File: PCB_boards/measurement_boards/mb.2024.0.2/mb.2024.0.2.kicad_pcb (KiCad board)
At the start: 2 copper layers, 247.8 x 124.2 mm, 121 parts, among them J1 DSP_out_12v_GND, J10 DSP+, J11 Screw_Terminal_VMN, J12 Conn_01x08_Female, J13 Connector_I2C_for_mux, J14 Conn_01x02_Female, J15 Conn_01x08_Female, J16 RX_bat, J17 DSP GND, J18 ELEC_M, J19 ELEC_N, J2 DPS5005_input_0_to_50V, J20 shunt +, J21 shunt -, J22 Conn_01x04_Female, J23 Conn_01x05_Female, J24 Connector_I2C_for_MC, J25 Conn_01x04_Female, J26 Conn_01x05_Female, J3 Screw_Terminal_AB, J4 Conn_01x08_Female, J5 Conn_01x04_Female, J6 Conn_01x08_Female, J7 Raspberry_Pi_2_3, J8 Connector_I2C_for_MCP23008, J9 TX_bat, K1 G5LE-1, K2 G5LE-1, K3 G5LE-1, K4 G5LE-1, K5 G5LE-1, K6 G5LE-1, Q1 ZVN4206ASTZ, Q2 ZVN4206ASTZ, Q3 ZVN4206ASTZ, Q4 ZVN4206ASTZ, Q5 ZVN4206ASTZ, Q6 ZVN4206ASTZ, U1 MCP23008-xP, U10 DG411xJ, U2 OP07, U3 24LC02, U4 1085, U5 1085, U6 OP07, U7 REF03GP, U8 MCP23008-xP, U9 OP07

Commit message: correction DPS, add dischage resistor, remove 63 warning on the schemtic, remove 7 errors in schematics change resistor designation, update pcb
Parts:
- removed C9: 10uF, Capacitor_THT:CP_Radial_D6.3mm_P2.50mm
- removed LED10-OHMPI-MEASURE: LED, LED_THT:LED_D4.0mm
- removed R11: 330 ohms, Resistor_THT:R_Axial_DIN0207_L6.3mm_D2.5mm_P7.62mm_Horizontal
- removed R21, R22: 4.7K, Resistor_THT:R_Axial_DIN0207_L6.3mm_D2.5mm_P7.62mm_Horizontal
- added C5: 10uF, Capacitor_THT:CP_Radial_D6.3mm_P2.50mm, F.Cu at (109.3, 81.5)
- added D9: 1N4001, Diode_THT:D_DO-41_SOD81_P10.16mm_Horizontal, F.Cu at (153.4, 127.3)
- added J27: Screw_Terminal_01x03, TerminalBlock:TerminalBlock_bornier-3_P5.08mm, F.Cu at (105.2, 51.1)
- added K7: G5LE-1, Relay_THT:Relay_SPDT_Omron-G5LE-1, F.Cu at (168.6, 132.1)
- added Q7: ZVN4206ASTZ, Package_TO_SOT_THT:TO-92L_Wide, F.Cu at (188.5, 135.9)
- added R8: 1k, Resistor_THT:R_Axial_DIN0207_L6.3mm_D2.5mm_P7.62mm_Horizontal, F.Cu at (156.7, 131.6)
- added R9: 100k, Resistor_THT:R_Axial_DIN0207_L6.3mm_D2.5mm_P7.62mm_Horizontal, F.Cu at (195.3, 142.5)
- J1: value DSP_out_12v_GND -> DPS_out_12v_GND
- J10: value DSP+ -> DPS+
- J12, J15, J4, J6: value Conn_01x08_Female -> Conn_01x08_Socket
- J14: value Conn_01x02_Female -> Conn_01x02_Socket
- J17: value DSP GND -> DPS GND
- J22: renamed from J5; value Conn_01x04_Female -> Conn_01x04_Socket
- J23: renamed from J26; value Conn_01x05_Female -> Conn_01x05_Socket
- J25: renamed from J22; value Conn_01x04_Female -> Conn_01x04_Socket
- J26: renamed from J23; value Conn_01x05_Female -> Conn_01x05_Socket
- J5: renamed from J25; value Conn_01x04_Female -> Conn_01x04_Socket
- moved J21 9.45 mm to (160.8, 141.0)
- renumbered D9 to D3, D10 to D4, D11 to D7, D12 to D8, LED11-OHMPI-STACK to LED11-OHMPI-STACK1, LED12-LOW-TX-BATTERY to LED12-LOW-TX-BATTERY1, LED9-OHMPI-RUN to LED9-OHMPI-RUN-1
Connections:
- net /Current_injection_and_measurement/Input_DSP_+_alim renamed /Current_injection_and_measurement/Input_DPS_+_alim
- net /Current_injection_and_measurement/Input_DSP_GND_alim renamed /Current_injection_and_measurement/Input_DPS_GND_alim
- net /Relay_switch_dsp/out_12v_DSP renamed /Relay_switch_DPS/out_12v_DPS
- net /Relay_switch_dsp/out_GND_DSP renamed /Relay_switch_DPS/out_GND_DPS
- U4 pad 1: unconnected-(U4-A3-Pad1) -> Net-(J27-Pin_1)
- U4 pad 2: unconnected-(U4-A2-Pad2) -> Net-(J27-Pin_2)
- U4 pad 3: unconnected-(U4-A1-Pad3) -> Net-(J27-Pin_3)
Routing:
- net Net-(J27-Pin_1): track 0.00 -> 43.5 mm
- net Net-(J27-Pin_2): track 0.00 -> 38.9 mm
- net Net-(D9-A): track 0.00 -> 35.8 mm
- net Net-(J27-Pin_3): track 0.00 -> 34.4 mm
- net /Current_injection_and_measurement/Input_DPS_+_alim: track 172.6 -> 199.9 mm
- net 5VD: track 554.0 -> 579.1 mm
- net GP5: track 62.8 -> 84.6 mm
- net Net-(K7-Pad1): track 0.00 -> 12.7 mm
- net GNDD: track 0.00 -> 9.59 mm
- net GP0: track 233.5 -> 225.8 mm
- net AN: track 51.9 -> 59.4 mm
- net GP1: track 282.5 -> 277.0 mm
- net Net-(LED10-OHMPI-MEASURE1-A): track 3.65 -> 0.00 mm
- net /Current_injection_and_measurement/Input_DPS_GND_alim: track 97.0 -> 99.9 mm
- net SDA2: vias 1 -> 2
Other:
- outline, holes or cut-outs redrawn
- board text added: "DPS Input"
- board text added: "DPS out +"
- board text added: "DPS out GND"
- board text removed: "DSP Input"
- board text removed: "Dps out +"
- board text removed: "Dps out GND"

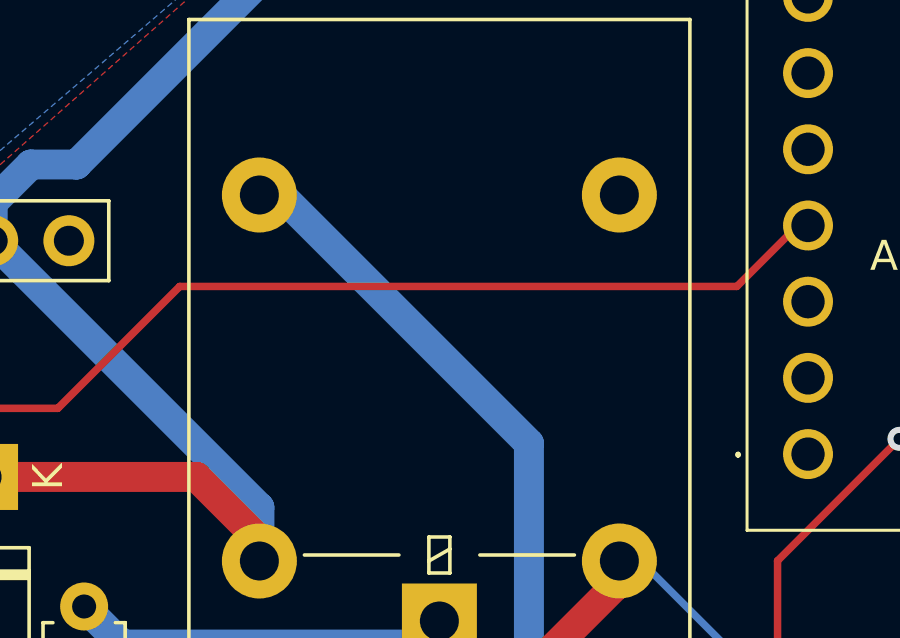
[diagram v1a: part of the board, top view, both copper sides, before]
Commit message: update measurement board
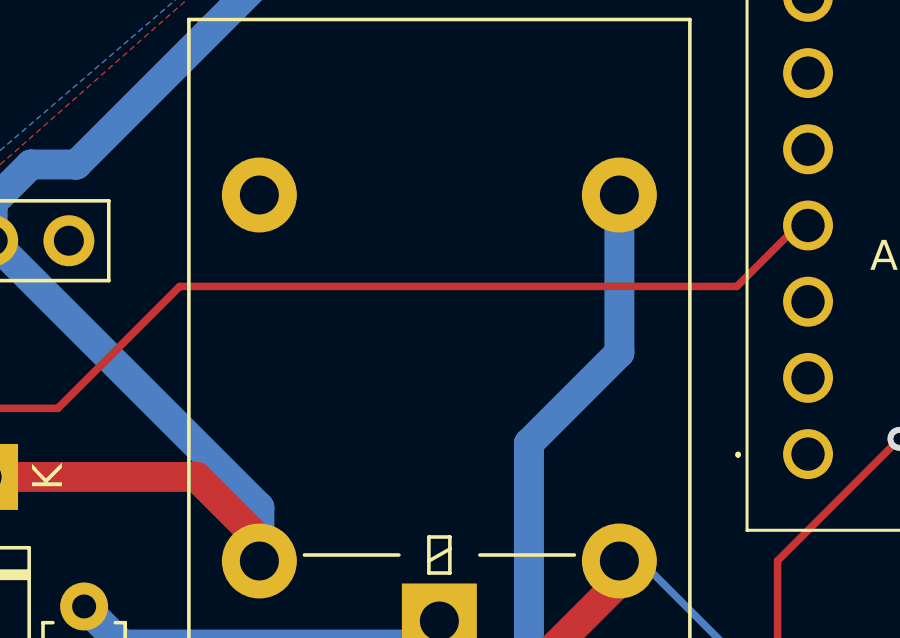
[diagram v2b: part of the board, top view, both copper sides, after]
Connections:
- K7 pad 3: unconnected-(K7-Pad3) -> /Current_injection_and_measurement/Input_DPS_+_alim
- K7 pad 4: /Current_injection_and_measurement/Input_DPS_+_alim -> unconnected-(K7-Pad4)
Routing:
- net /Current_injection_and_measurement/Input_DPS_+_alim: track 199.9 -> 197.0 mm
- net unconnected-(K7-Pad4): track 0.00 -> 0.71 mm
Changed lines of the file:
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@@
   (net 162 "/Current_injection_and_measurement/Input_DPS_GND_alim")
   (net 163 "Net-(K7-Pad1)")
-  (net 164 "unconnected-(K7-Pad3)")
-  (net 165 "Net-(J27-Pin_1)")
-  (net 166 "Net-(J27-Pin_2)")
-  (net 167 "Net-(J27-Pin_3)")
+  (net 164 "Net-(J27-Pin_1)")
+  (net 165 "Net-(J27-Pin_2)")
+  (net 166 "Net-(J27-Pin_3)")
+  (net 167 "unconnected-(K7-Pad4)")
   (footprint "Connector_PinHeader_2.54mm:PinHeader_1x01_P2.54mm_Vertical" (layer "F.Cu")
     (at 26.162 77.978)
@@
       (stroke (width 0.1) (type solid)) (layer "F.Fab"))
     (pad "1" thru_hole rect (at 0 0) (size 3 3) (drill 1.52) (layers "*.Cu" "*.Mask")
-      (net 165 "Net-(J27-Pin_1)") (pinfunction "Pin_1") (pintype "passive"))
+      (net 164 "Net-(J27-Pin_1)") (pinfunction "Pin_1") (pintype "passive"))
     (pad "2" thru_hole circle (at 5.08 0) (size 3 3) (drill 1.52) (layers "*.Cu" "*.Mask")
-      (net 166 "Net-(J27-Pin_2)") (pinfunction "Pin_2") (pintype "passive"))
+      (net 165 "Net-(J27-Pin_2)") (pinfunction "Pin_2") (pintype "passive"))
     (pad "3" thru_hole circle (at 10.16 0) (size 3 3) (drill 1.52) (layers "*.Cu" "*.Mask")
-      (net 167 "Net-(J27-Pin_3)") (pinfunction "Pin_3") (pintype "passive"))
+      (net 166 "Net-(J27-Pin_3)") (pinfunction "Pin_3") (pintype "passive"))
     (model "${KICAD6_3DMODEL_DIR}/TerminalBlock.3dshapes/TerminalBlock_bornier-3_P5.08mm.wrl"
       (offset (xyz 5.079999924 0 0))
@@
     (property "Arrow Part Number" "ZVN4206ASTZ")
     (property "Arrow Price/Stock" "https://www.arrow.com/en/products/zvn4206astz/diodes-incorporated?region=nac")
-    (property "Description" "N-Channel 60 V 600mA (Ta) 700mW (Ta) Through Hole E-Line (TO-92 compatible)")
+    (property "Description" "Transistor JFET - TO shape - relay activation")
     (property "Height" "4.01")
     (property "Manufacturer_Name" "Diodes Incorporated")
@@
       (net 23 "Net-(D9-A)") (pintype "passive"))
     (pad "3" thru_hole oval (at -6 14.2 180) (size 2.5 2.5) (drill 1.3) (layers "*.Cu" "*.Mask")
-      (net 164 "unconnected-(K7-Pad3)") (pintype "passive+no_connect"))
-    (pad "4" thru_hole oval (at 6 14.2 180) (size 2.5 2.5) (drill 1.3) (layers "*.Cu" "*.Mask")
       (net 161 "/Current_injection_and_measurement/Input_DPS_+_alim") (pintype "passive"))
+    (pad "4" thru_hole oval (at 6 14.2 180) (size 2.5 2.5) (drill 1.3) (layers "*.Cu" "*.Mask")
+      (net 167 "unconnected-(K7-Pad4)") (pintype "passive+no_connect"))
     (pad "5" thru_hole oval (at 6 2 180) (size 2.5 2.5) (drill 1.3) (layers "*.Cu" "*.Mask")
       (net 1 "5VD") (pintype "passive"))
@@
       (stroke (width 0.2) (type solid)) (layer "F.Fab"))
     (pad "1" thru_hole circle (at 0 0 270) (size 1.665 1.665) (drill 1.11) (layers "*.Cu" "*.Mask")
-      (net 165 "Net-(J27-Pin_1)") (pinfunction "A3") (pintype "passive"))
+      (net 164 "Net-(J27-Pin_1)") (pinfunction "A3") (pintype "passive"))
     (pad "2" thru_hole circle (at -2.54 0 270) (size 1.665 1.665) (drill 1.11) (layers "*.Cu" "*.Mask")
-      (net 166 "Net-(J27-Pin_2)") (pinfunction "A2") (pintype "passive"))
+      (net 165 "Net-(J27-Pin_2)") (pinfunction "A2") (pintype "passive"))
     (pad "3" thru_hole circle (at -5.08 0 270) (size 1.665 1.665) (drill 1.11) (layers "*.Cu" "*.Mask")
-      (net 167 "Net-(J27-Pin_3)") (pinfunction "A1") (pintype "passive"))
+      (net 166 "Net-(J27-Pin_3)") (pinfunction "A1") (pintype "passive"))
     (pad "4" thru_hole circle (at -7.62 0 270) (size 1.665 1.665) (drill 1.11) (layers "*.Cu" "*.Mask")
       (net 22 "Net-(D5-A)") (pinfunction "A0") (pintype "passive"))
@@
     (property "Arrow Part Number" "ZVN4206ASTZ")
     (property "Arrow Price/Stock" "https://www.arrow.com/en/products/zvn4206astz/diodes-incorporated?region=nac")
-    (property "Description" "N-Channel 60 V 600mA (Ta) 700mW (Ta) Through Hole E-Line (TO-92 compatible)")
+    (property "Description" "Transistor JFET - TO shape - relay activation")
     (property "Height" "4.01")
     (property "Manufacturer_Name" "Diodes Incorporated")
@@
   (segment (start 171.545 141) (end 177 141) (width 1) (layer "F.Cu") (net 161))
   (segment (start 76.2 138.1675) (end 72.6525 138.1675) (width 2) (layer "B.Cu") (net 161))
-  (segment (start 163.268 117.856) (end 162.56 117.856) (width 1) (layer "B.Cu") (net 161))
   (segment (start 63.5 134.62) (end 60.96 132.08) (width 2) (layer "B.Cu") (net 161))
   (segment (start 60.96 132.08) (end 39.37 132.08) (width 2) (layer "B.Cu") (net 161))
-  (segment (start 171.545 126.133) (end 163.268 117.856) (width 1) (layer "B.Cu") (net 161))
   (segment (start 65.11 138.77) (end 63.5 137.16) (width 2) (layer "B.Cu") (net 161))
   (segment (start 39.37 132.08) (end 35.56 135.89) (width 2) (layer "B.Cu") (net 161))
+  (segment (start 174.56 123.118) (end 174.56 117.856) (width 1) (layer "B.Cu") (net 161))
   (segment (start 63.5 137.16) (end 63.5 134.62) (width 2) (layer "B.Cu") (net 161))
   (segment (start 35.56 135.89) (end 35.56 138.1675) (width 2) (layer "B.Cu") (net 161))
@@
   (segment (start 65.42727 138.77) (end 65.11 138.77) (width 2) (layer "B.Cu") (net 161))
   (segment (start 171.545 141) (end 171.545 126.133) (width 1) (layer "B.Cu") (net 161))
+  (segment (start 171.545 126.133) (end 174.56 123.118) (width 1) (layer "B.Cu") (net 161))
   (segment (start 119.475 126.395) (end 123.445 126.395) (width 2) (layer "F.Cu") (net 162))
   (segment (start 124.43 127.38) (end 124.43 144.38) (width 2) (layer "F.Cu") (net 162))
@@
   (segment (start 167.774 132.842) (end 168.56 132.056) (width 1) (layer "B.Cu") (net 163))
   (segment (start 156.718 131.572) (end 157.988 132.842) (width 1) (layer "B.Cu") (net 163))
-  (segment (start 119.692 72.136) (end 108.575 61.019) (width 0.25) (layer "B.Cu") (net 165))
-  (segment (start 122.6 87.376) (end 119.692 84.468) (width 0.25) (layer "B.Cu") (net 165))
-  (segment (start 119.692 84.468) (end 119.692 72.136) (width 0.25) (layer "B.Cu") (net 165))
-  (segment (start 108.575 61.019) (end 108.575 54.473) (width 0.25) (layer "B.Cu") (net 165))
-  (segment (start 108.575 54.473) (end 105.156 51.054) (width 0.25) (layer "B.Cu") (net 165))
-  (segment (start 120.142 71.882) (end 120.142 82.378) (width 0.25) (layer "B.Cu") (net 166))
-  (segment (start 110.236 61.976) (end 120.142 71.882) (width 0.25) (layer "B.Cu") (net 166))
-  (segment (start 120.142 82.378) (end 122.6 84.836) (width 0.25) (layer "B.Cu") (net 166))
-  (segment (start 110.236 51.054) (end 110.236 61.976) (width 0.25) (layer "B.Cu") (net 166))
-  (segment (start 115.316 51.054) (end 115.316 66.294) (width 0.25) (layer "B.Cu") (net 167))
-  (segment (start 115.316 66.294) (end 120.396 71.374) (width 0.25) (layer "B.Cu") (net 167))
-  (segment (start 120.65 71.374) (end 120.65 80.346) (width 0.25) (layer "B.Cu") (net 167))
-  (segment (start 120.396 71.374) (end 120.65 71.374) (width 0.25) (layer "B.Cu") (net 167))
-  (segment (start 120.65 80.346) (end 122.6 82.296) (width 0.25) (layer "B.Cu") (net 167))
+  (segment (start 119.692 72.136) (end 108.575 61.019) (width 0.25) (layer "B.Cu") (net 164))
+  (segment (start 122.6 87.376) (end 119.692 84.468) (width 0.25) (layer "B.Cu") (net 164))
+  (segment (start 119.692 84.468) (end 119.692 72.136) (width 0.25) (layer "B.Cu") (net 164))
+  (segment (start 108.575 61.019) (end 108.575 54.473) (width 0.25) (layer "B.Cu") (net 164))
+  (segment (start 108.575 54.473) (end 105.156 51.054) (width 0.25) (layer "B.Cu") (net 164))
+  (segment (start 120.142 71.882) (end 120.142 82.378) (width 0.25) (layer "B.Cu") (net 165))
+  (segment (start 110.236 61.976) (end 120.142 71.882) (width 0.25) (layer "B.Cu") (net 165))
+  (segment (start 120.142 82.378) (end 122.6 84.836) (width 0.25) (layer "B.Cu") (net 165))
+  (segment (start 110.236 51.054) (end 110.236 61.976) (width 0.25) (layer "B.Cu") (net 165))
+  (segment (start 115.316 51.054) (end 115.316 66.294) (width 0.25) (layer "B.Cu") (net 166))
+  (segment (start 115.316 66.294) (end 120.396 71.374) (width 0.25) (layer "B.Cu") (net 166))
+  (segment (start 120.65 71.374) (end 120.65 80.346) (width 0.25) (layer "B.Cu") (net 166))
+  (segment (start 120.396 71.374) (end 120.65 71.374) (width 0.25) (layer "B.Cu") (net 166))
+  (segment (start 120.65 80.346) (end 122.6 82.296) (width 0.25) (layer "B.Cu") (net 166))
+  (segment (start 163.268 117.856) (end 162.56 117.856) (width 1) (layer "B.Cu") (net 167))
   (zone (net 2) (net_name "GNDD") (layer "F.Cu") (hatch edge 0.508)
     (connect_pads (clearance 0.508))

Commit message: update measurement board
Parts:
- removed the C5 at (109.3, 81.5)
- removed the D9 at (153.4, 127.3)
- removed J27: Screw_Terminal_01x03, TerminalBlock:TerminalBlock_bornier-3_P5.08mm
- removed K7: G5LE-1, Relay_THT:Relay_SPDT_Omron-G5LE-1
- removed Q7: ZVN4206ASTZ, Package_TO_SOT_THT:TO-92L_Wide
- removed R8: 1k, Resistor_THT:R_Axial_DIN0207_L6.3mm_D2.5mm_P7.62mm_Horizontal
- removed R9: 100k, Resistor_THT:R_Axial_DIN0207_L6.3mm_D2.5mm_P7.62mm_Horizontal
- added C9: 10uF, Capacitor_THT:CP_Radial_D6.3mm_P2.50mm, F.Cu at (109.2, 81.5)
- added LED10-OHMPI-MEASURE: LED, LED_THT:LED_D4.0mm, F.Cu at (235.0, 130.0)
- added R11: 330 ohms, Resistor_THT:R_Axial_DIN0207_L6.3mm_D2.5mm_P7.62mm_Horizontal, F.Cu at (235.0, 116.2)
- added R21: 4.7K, Resistor_THT:R_Axial_DIN0207_L6.3mm_D2.5mm_P7.62mm_Horizontal, F.Cu at (111.5, 58.9)
- added R22: 4.7K, Resistor_THT:R_Axial_DIN0207_L6.3mm_D2.5mm_P7.62mm_Horizontal, F.Cu at (116.6, 58.9)
- J1: value DPS_out_12v_GND -> DSP_out_12v_GND
- J10: value DPS+ -> DSP+
- J12, J15, J4, J6: value Conn_01x08_Socket -> Conn_01x08_Female
- J14: value Conn_01x02_Socket -> Conn_01x02_Female
- J17: value DPS GND -> DSP GND
- J22: renamed from J25; value Conn_01x04_Socket -> Conn_01x04_Female
- J23: renamed from J26; value Conn_01x05_Socket -> Conn_01x05_Female
- J25: renamed from J5; value Conn_01x04_Socket -> Conn_01x04_Female
- J26: renamed from J23; value Conn_01x05_Socket -> Conn_01x05_Female
- J5: renamed from J22; value Conn_01x04_Socket -> Conn_01x04_Female
- moved J21 9.45 mm to (166.4, 133.3)
- renumbered D4 to D10, D7 to D11, D8 to D12, D3 to D9, LED11-OHMPI-STACK1 to LED11-OHMPI-STACK, LED12-LOW-TX-BATTERY1 to LED12-LOW-TX-BATTERY, LED9-OHMPI-RUN-1 to LED9-OHMPI-RUN
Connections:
- net /Current_injection_and_measurement/Input_DPS_+_alim renamed /Current_injection_and_measurement/Input_DSP_+_alim
- net /Current_injection_and_measurement/Input_DPS_GND_alim renamed /Current_injection_and_measurement/Input_DSP_GND_alim
- net /Relay_switch_DPS/out_12v_DPS renamed /Relay_switch_dsp/out_12v_DSP
- net /Relay_switch_DPS/out_GND_DPS renamed /Relay_switch_dsp/out_GND_DSP
- U4 pad 1: Net-(J27-Pin_1) -> unconnected-(U4-A3-Pad1)
- U4 pad 2: Net-(J27-Pin_2) -> unconnected-(U4-A2-Pad2)
- U4 pad 3: Net-(J27-Pin_3) -> unconnected-(U4-A1-Pad3)
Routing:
- net Net-(J27-Pin_1): track 43.5 -> 0.00 mm
- net Net-(J27-Pin_2): track 38.9 -> 0.00 mm
- net Net-(D9-A) (its old number): track 35.8 -> 0.00 mm
- net Net-(J27-Pin_3): track 34.4 -> 0.00 mm
- net 5VD: track 579.1 -> 554.0 mm
- net /Current_injection_and_measurement/Input_DSP_+_alim: track 197.0 -> 172.6 mm
- net GP5: track 84.6 -> 62.8 mm
- net Net-(K7-Pad1): track 12.7 -> 0.00 mm
- net GNDD: track 9.59 -> 0.00 mm
- net GP0: track 225.8 -> 233.5 mm
- net AN: track 59.4 -> 51.9 mm
- net GP1: track 277.0 -> 282.5 mm
- net Net-(LED10-OHMPI-MEASURE1-A): track 0.00 -> 3.65 mm
- net /Current_injection_and_measurement/Input_DSP_GND_alim: track 99.9 -> 97.0 mm
- net unconnected-(K7-Pad4): track 0.71 -> 0.00 mm
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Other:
- outline, holes or cut-outs redrawn
- board text added: "DSP Input"
- board text added: "Dps out +"
- board text added: "Dps out GND"
- board text removed: "DPS Input"
- board text removed: "DPS out +"
- board text removed: "DPS out GND"
